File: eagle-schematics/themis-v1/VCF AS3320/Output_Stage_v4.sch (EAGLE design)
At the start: 43 parts

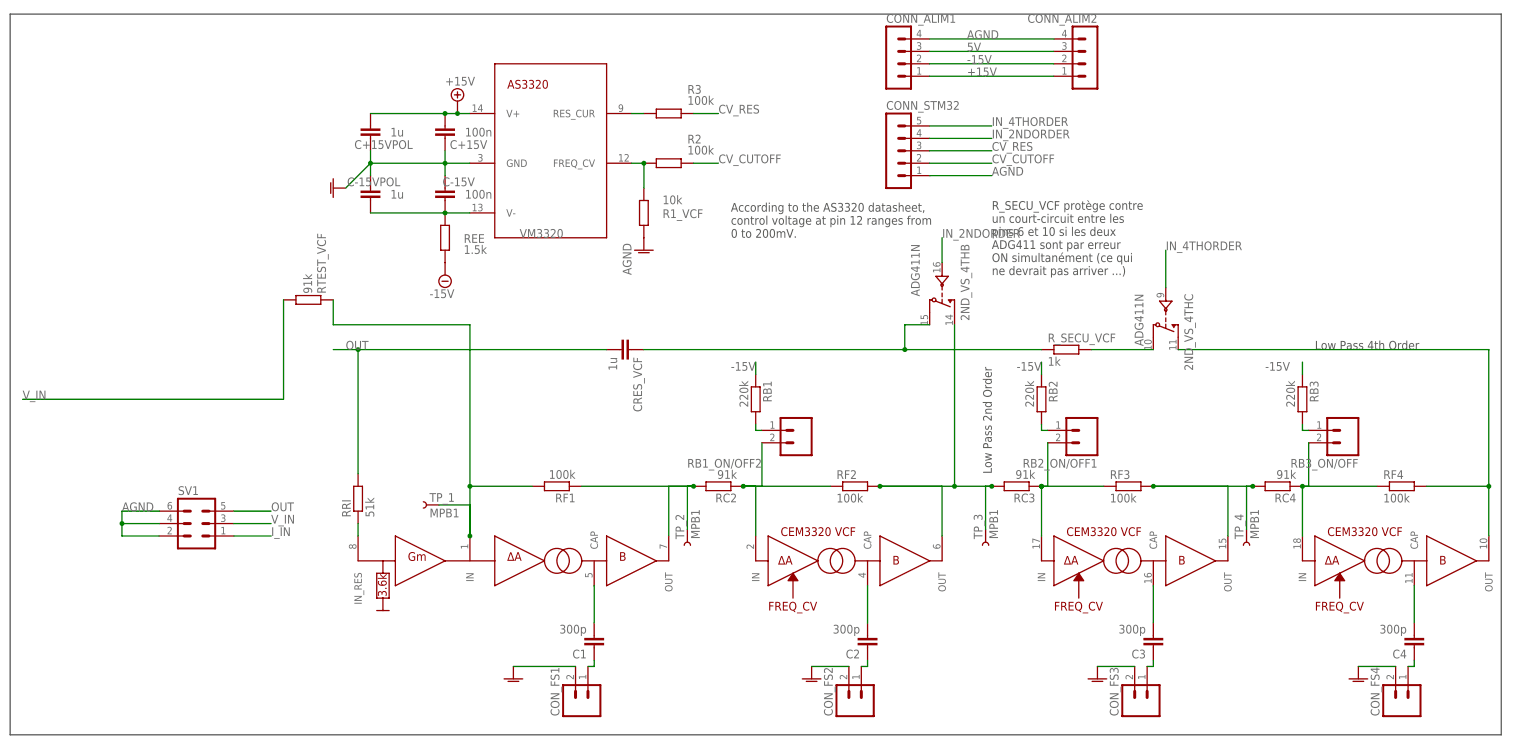
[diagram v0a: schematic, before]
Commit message: Add files via upload
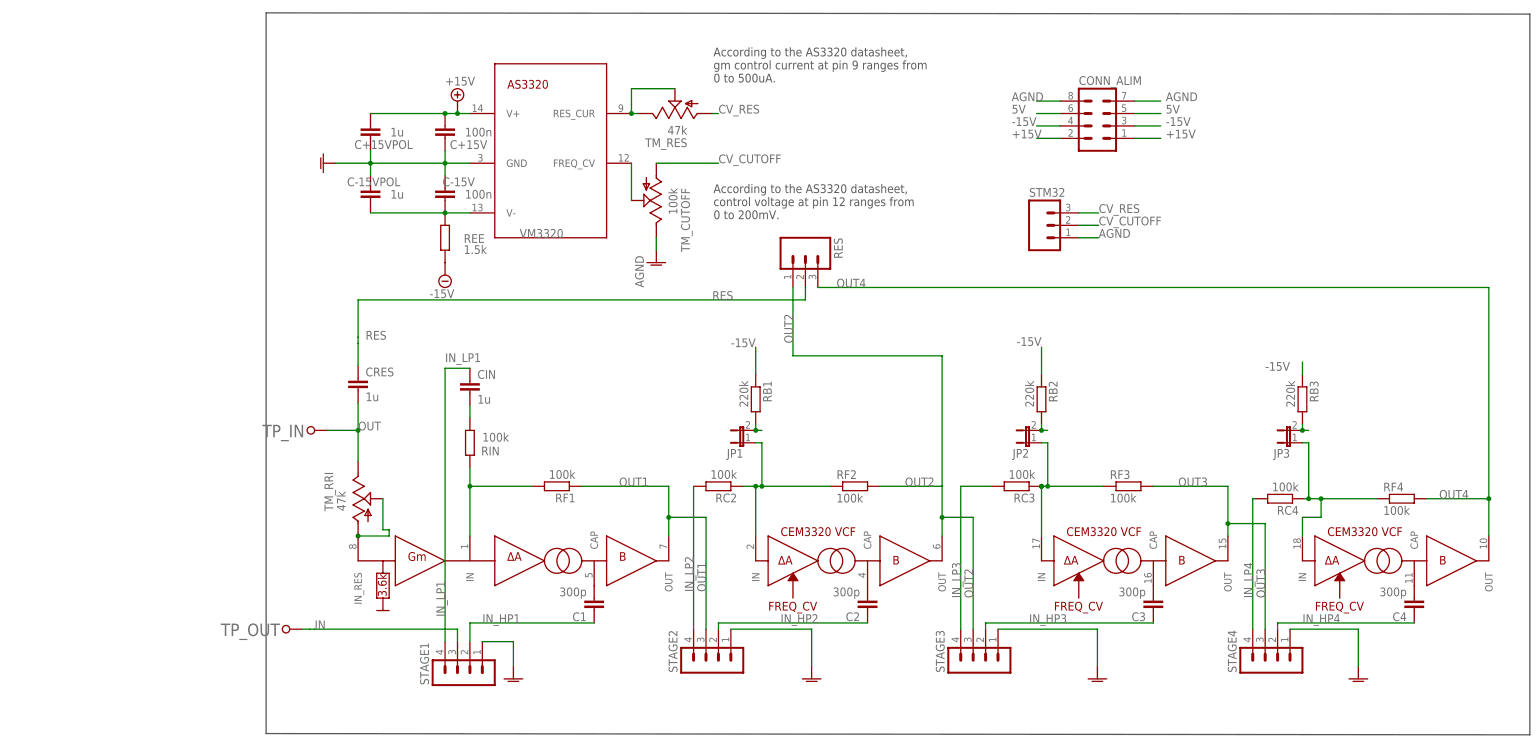
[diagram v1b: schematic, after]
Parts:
- removed 2ND_VS_4TH: ADG411N, analog-devices:ADG411N
- removed CONN_ALIM1, CONN_ALIM2: (no value), con-lstb:MA04-1
- removed CONN_STM32: (no value), con-lstb:MA05-1
- removed CON_FS1, CON_FS2, CON_FS3, CON_FS4, RB1_ON/OFF2, RB2_ON/OFF1, RB3_ON/OFF: (no value), con-amp-quick:MA02
- removed CRES_VCF: 1u, rcl:C-EU075-032X103
- removed R1_VCF: 10k, rcl:R-EU_0204/7
- removed R2, R3: 100k, rcl:R-EU_0204/7
- removed RRI: 51k, rcl:R-EU_0207/10
- removed RTEST_VCF: 91k, rcl:R-EU_0207/10
- removed R_SECU_VCF: 1k, rcl:R-EU_0204/7
- removed SV1: (no value), con-lstb:MA03-2
- removed TP_1, TP_2, TP_3, TP_4: MPB1, con-hirschmann:MPB1
- added CIN, CRES: 1u, rcl:C-EU050-030X075
- added CONN_ALIM: (no value), con-lstb:MA04-2
- added JP1, JP2, JP3: (no value), jumper:JP1E
- added RES, STM32: (no value), con-amp-quick:MA03
- added RIN: 100k, rcl:R-EU_0204/7
- added STAGE1, STAGE2, STAGE3, STAGE4: (no value), con-lstb:MA04-1
- added TM_CUTOFF: 100k, adafruit:TRIM
- added TM_RES, TM_RRI: 47k, adafruit:TRIM
- added TP_IN, TP_OUT: (no value), 6P1_EVB:TESTPOINT
- C+15V, C+15VPOL, C-15V, C-15VPOL: device rcl:C-EU075-032X103 -> rcl:C-EU050-050X075
- C1, C3, C4: device rcl:C-EU075-032X103 -> rcl:C-EU050-030X075
- RB1, RF1, RF3: device rcl:R-EU_0207/10 -> rcl:R-EU_0204/7
- RC2, RC3, RC4: value 91k -> 100k
- REE: device rcl:R-EU_0207/10 -> rcl:R-EU_0207/7
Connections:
- removed net IN_2NDORDER: 2ND_VS_4THB.IN, CONN_STM32.4
- removed net IN_4THORDER: 2ND_VS_4THC.IN, CONN_STM32.5
- removed net I_IN: SV1.1
- removed net N$2: C1.1, CON_FS1.1
- removed net N$3: C2.1, CON_FS2.1
- removed net N$4: C3.1, CON_FS3.1
- removed net N$57: RC2.2, RF1.1, TP_2.1, VCFOTA$1.OUT
- removed net N$58: 2ND_VS_4THB.D, CRES_VCF.1, R_SECU_VCF.1
- removed net N$6: C4.1, CON_FS4.1
- removed net N$65: 2ND_VS_4THB.S, RC3.2, RF2.2, TP_3.1, VCFOTA$2.OUT
- removed net N$69: 2ND_VS_4THC.S, RF4.2, VCFOTA$3.OUT
- removed net N$73: 2ND_VS_4THC.D, R_SECU_VCF.2
- removed net N$82: RC4.2, RF3.2, TP_4.1, VCFOTA$4.OUT
- removed net N$83: RB3_ON/OFF.2, RC4.1, RF4.1, VCFOTA$3.IN
- removed net V_IN: RTEST_VCF.1, SV1.3
- new net IN: STAGE1.3, TP_OUT.P$1
- new net IN_HP1: C1.1, STAGE1.2
- new net IN_HP2: C2.1, STAGE2.2
- new net IN_HP3: C3.1, STAGE3.2
- new net IN_HP4: C4.1, STAGE4.2
- new net IN_LP1: CIN.1, STAGE1.4
- new net IN_LP2: RC2.2, STAGE2.4
- new net IN_LP3: RC3.2, STAGE3.4
- new net IN_LP4: RC4.2, STAGE4.4
- new net N$15: JP3.1, RC4.1, RF4.1, VCFOTA$3.IN
- new net N$17: CIN.2, RIN.1
- new net OUT1: RF1.1, STAGE2.3, VCFOTA$1.OUT
- new net OUT2: RES.1, RF2.2, STAGE3.3, VCFOTA$2.OUT
- new net OUT3: RF3.2, STAGE4.3, VCFOTA$4.OUT
- new net OUT4: RES.3, RF4.2, VCFOTA$3.OUT
- new net RES: CRES.1, RES.2
- net +15V: now also CONN_ALIM.1, CONN_ALIM.2; no longer CONN_ALIM1.1, CONN_ALIM2.1
- net -15V: now also CONN_ALIM.3, CONN_ALIM.4; no longer CONN_ALIM1.2, CONN_ALIM2.2
- net 5V: now also CONN_ALIM.5, CONN_ALIM.6; no longer CONN_ALIM1.3, CONN_ALIM2.3
- net AGND: now also CONN_ALIM.7, CONN_ALIM.8, STAGE1.1, STAGE2.1, STAGE3.1, STAGE4.1, STM32.1, TM_CUTOFF.E; no longer CONN_ALIM1.4, CONN_ALIM2.4, CONN_STM32.1, CON_FS1.2, CON_FS2.2, CON_FS3.2, CON_FS4.2, R1_VCF.2, SV1.2, SV1.4, SV1.6
- net CV_CUTOFF: now also STM32.2, TM_CUTOFF.A; no longer CONN_STM32.2, R2.2
- net CV_RES: now also STM32.3, TM_RES.A; no longer CONN_STM32.3, R3.2
- net N$10: now also JP3.2; no longer RB3_ON/OFF.1
- net N$37: now also TM_CUTOFF.S; no longer R1_VCF.1, R2.1
- net N$62: now also JP1.1; no longer RB1_ON/OFF2.2
- net N$7: now also JP1.2; no longer RB1_ON/OFF2.1
- net N$72: now also JP2.1; no longer RB2_ON/OFF1.2
- net N$86: now also TM_RRI.A, TM_RRI.S; no longer RRI.1
- net N$87: now also TM_RES.E, TM_RES.S; no longer R3.1
- net N$9: now also JP2.2; no longer RB2_ON/OFF1.1
- net OUT: now also CRES.2, TM_RRI.E, TP_IN.P$1; no longer CRES_VCF.2, RRI.2, SV1.5
- net VCF_IN: now also RIN.2; no longer RTEST_VCF.2, TP_1.1
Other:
- note added: "According to the AS3320 datasheet, gm control current at pin 9 ranges from 0 to 500uA."
- note removed: "Low Pass 2nd Order"
- note removed: "Low Pass 4th Order"
- note removed: "R_SECU_VCF protège contre un court-circuit entre les pins 6 et 10 si les deux ADG411 sont par erreur ON simultanément (ce qui ne devrait pas arriver ...)"
- moved on the sheet: C1, C2, C3, C4, RC4, RF4
